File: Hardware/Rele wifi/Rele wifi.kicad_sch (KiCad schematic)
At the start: 19 parts, among them J1 Screw_Terminal_01x02, J2 Screw_Terminal_01x02, J3 Conn_01x15_Pin, J4 Conn_01x15_Pin, K1 G5LE-1, Q1 BF457, Q2 BF457, SW1 SW_Push, U1 PC817

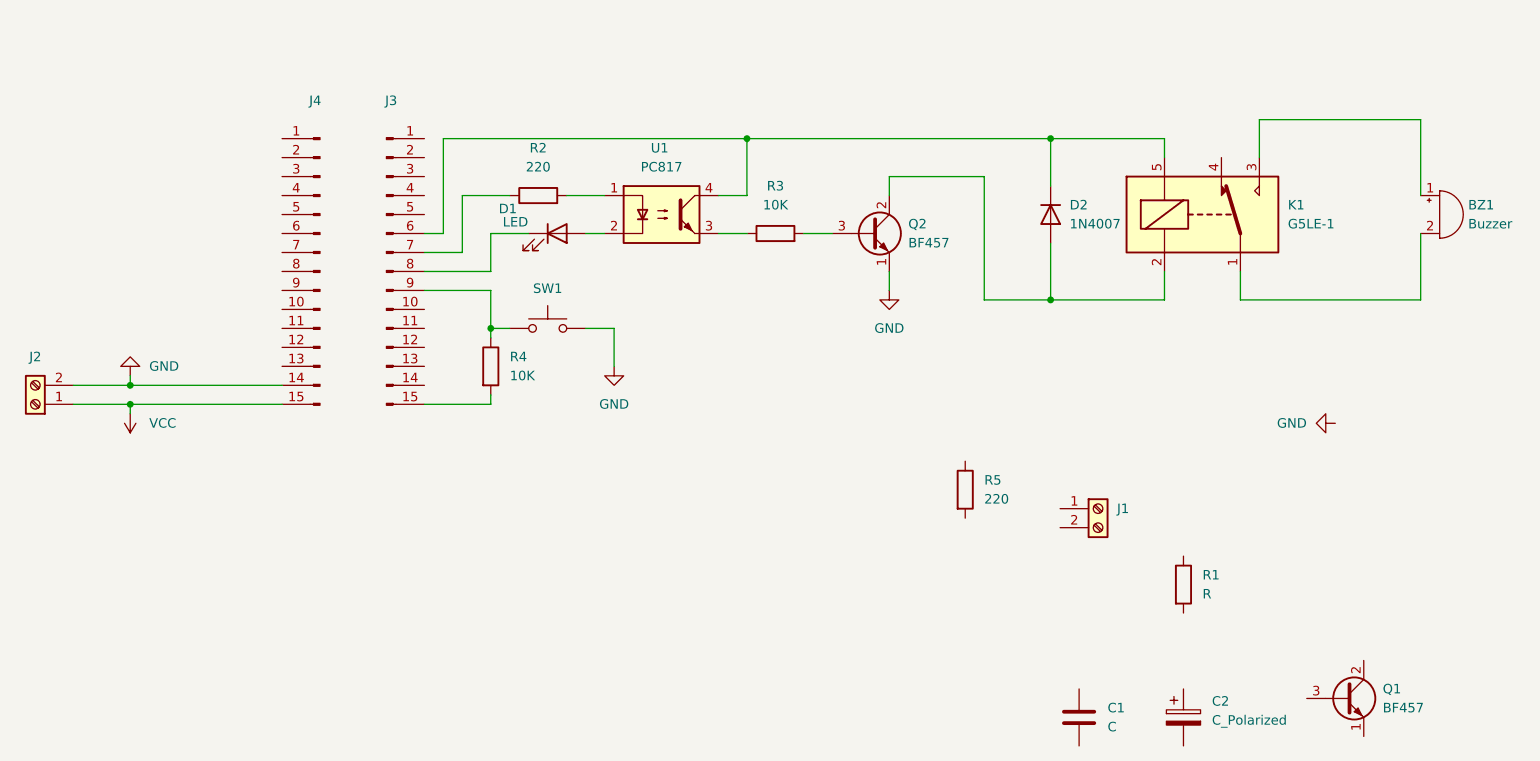
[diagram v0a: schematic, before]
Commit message: placa
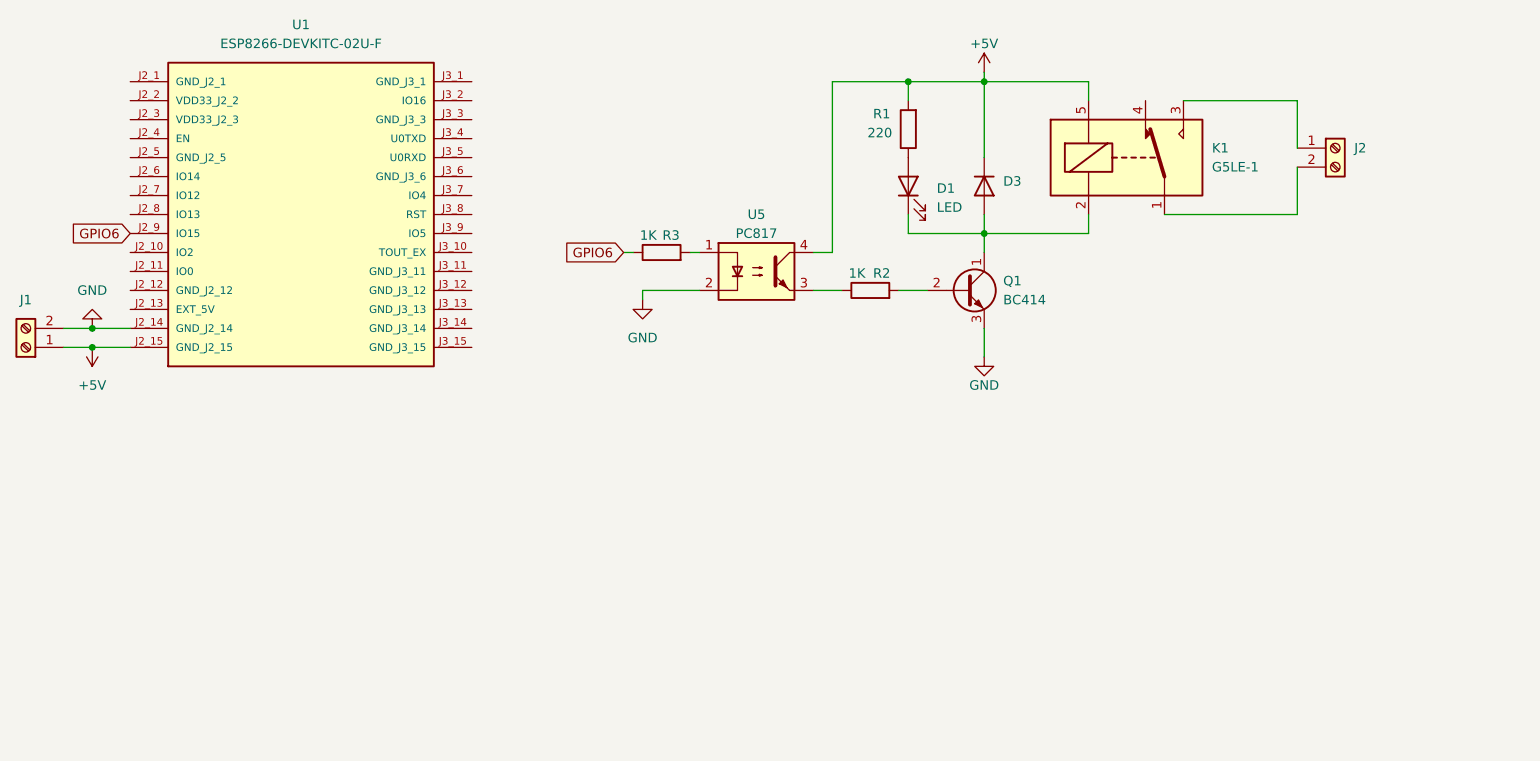
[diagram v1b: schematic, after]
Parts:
- removed BZ1: Buzzer, Buzzer_Beeper:Buzzer_12x9.5RM7.6, symbol Device:Buzzer
- removed C1: C, Capacitor_SMD:C_0201_0603Metric, symbol Device:C
- removed C2: C_Polarized, Capacitor_THT:CP_Radial_D5.0mm_P2.50mm, symbol Device:C_Polarized
- removed D2: 1N4007, Diode_THT:D_DO-41_SOD81_P10.16mm_Horizontal, symbol Diode:1N4007
- removed J3, J4: Conn_01x15_Pin, Connector_PinHeader_1.00mm:PinHeader_1x15_P1.00mm_Vertical, symbol Connector:Conn_01x15_Pin
- removed Q1, Q2: BF457, Package_TO_SOT_THT:TO-126-3_Vertical, symbol Transistor_BJT:BF457
- removed R4: 10K, Resistor_SMD:R_0201_0603Metric, symbol Device:R
- removed R5: 220, Resistor_SMD:R_0201_0603Metric, symbol Device:R
- removed SW1: SW_Push, Button_Switch_THT:SW_PUSH_6mm_H5mm, symbol Switch:SW_Push
- removed U1: PC817, Package_DIP:DIP-4_W7.62mm, symbol Isolator:PC817
- added D3: 1N4007, Diode_SMD:D_0805_2012Metric, symbol local_lib:1N4007
- added Q1: BC414, Package_TO_SOT_THT:TO-92_Inline, symbol Transistor_BJT:BC414
- added U1: ESP8266-DEVKITC-02U-F, esp32:ESP8266NA, symbol ESP8266-DEVKITC-02U-F:ESP8266-DEVKITC-02U-F
- added U5: PC817, Package_DIP:DIP-4_W7.62mm, symbol local_lib:PC817
- D1: footprint LED_THT:LED_D3.0mm -> LED_THT:LED_D3.0mm_Clear
- R1: value R -> 220; footprint Resistor_SMD:R_0201_0603Metric -> Resistor_SMD:R_0805_2012Metric
- R2: value 220 -> 1K; footprint Resistor_SMD:R_0201_0603Metric -> Resistor_SMD:R_0805_2012Metric
- R3: value 10K -> 1K; footprint Resistor_SMD:R_0201_0603Metric -> Resistor_SMD:R_0805_2012Metric
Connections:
- net VCC is gone; now on an unnamed net: J2.1 (Pin_1)
- net GND: now also J1.2 (Pin_2), Q1.3 (E), U1.J2_14 (GND_J2_14), U5.2; no longer J2.2 (Pin_2)
- net +5V: now reaches K1.5
- net +5V: now also J1.1 (Pin_1), R1.2, D3.1 (K), U1.J2_15 (GND_J2_15), U5.4
- net at K1.2: now also D1.1 (K), D3.2 (A), Q1.1 (C)
- net at R2.1: now also U5.3
- net at R2.2: now also Q1.2 (B)
- net at K1.1: now also J2.2 (Pin_2)
- net at D1.2 (A): now also R1.1
- net GPIO6: now reaches R3.1
- net GPIO6: now also U1.J2_9 (IO15)
- net at R3.2: now also U5.1
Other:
- moved on the sheet: K1
